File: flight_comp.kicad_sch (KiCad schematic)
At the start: 1 part, among them U1 STM32F405RGTx

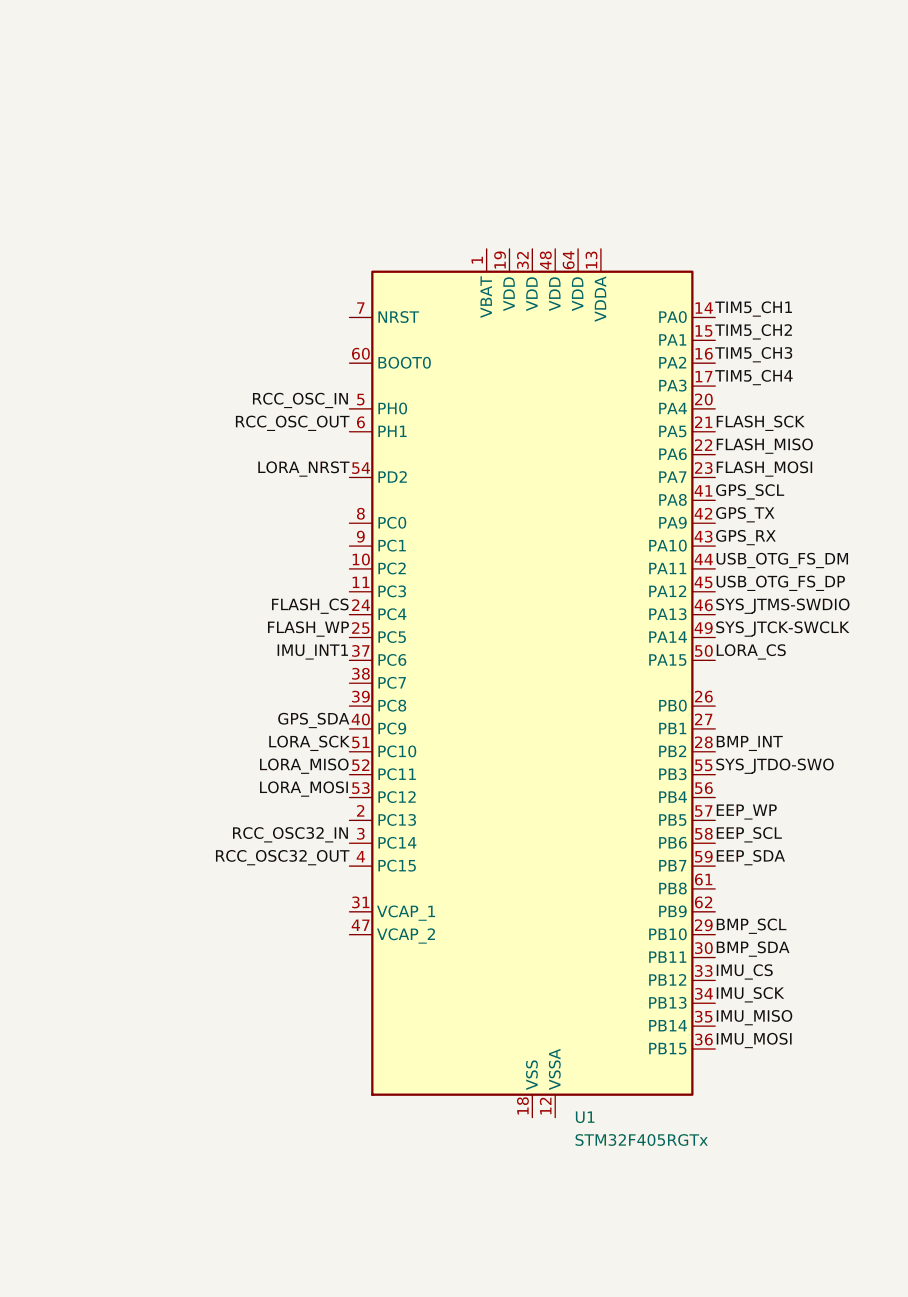
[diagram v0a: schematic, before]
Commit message: Sensors added
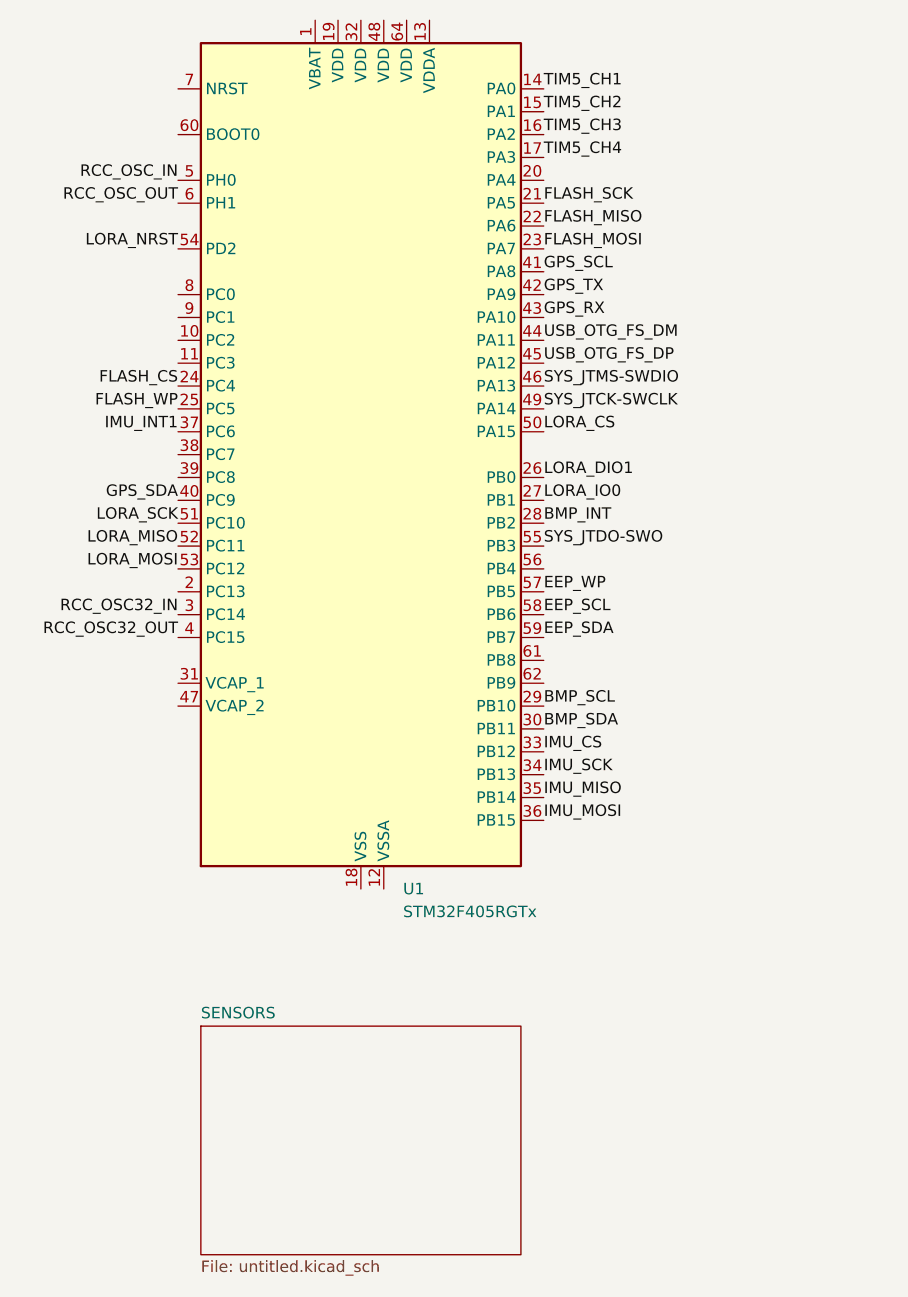
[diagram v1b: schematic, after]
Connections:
- net LORA_DIO1: now reaches U1.26 (PB0)
- net LORA_IO0: now reaches U1.27 (PB1)
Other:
- added sheet SENSORS (untitled.kicad_sch)
- moved on the sheet: U1
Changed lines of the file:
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@@
 	(paper "A4")
 	(label "TIM5_CH1"
-		(at 163.83 62.23 0)
+		(at 144.78 36.83 0)
+		(effects
+			(font
+				(size 1.27 1.27)
+			)
+			(justify left bottom)
+		)
+	)
+	(label "LORA_DIO1"
+		(at 144.78 80.01 0)
 		(effects
 			(font
@@
 	)
 	(label "EEP_SCL"
-		(at 163.83 120.65 0)
+		(at 144.78 95.25 0)
 		(effects
 			(font
@@
 	)
 	(label "TIM5_CH2"
-		(at 163.83 64.77 0)
+		(at 144.78 39.37 0)
 		(effects
 			(font
@@
 	)
 	(label "IMU_SCK"
-		(at 163.83 138.43 0)
+		(at 144.78 113.03 0)
 		(effects
 			(font
@@
 	)
 	(label "LORA_NRST"
-		(at 123.19 80.01 180)
+		(at 104.14 54.61 180)
 		(effects
 			(font
@@
 	)
 	(label "GPS_SDA"
-		(at 123.19 107.95 180)
+		(at 104.14 82.55 180)
 		(effects
 			(font
@@
 	)
 	(label "LORA_MOSI"
-		(at 123.19 115.57 180)
+		(at 104.14 90.17 180)
 		(effects
 			(font
@@
 	)
 	(label "USB_OTG_FS_DM"
-		(at 163.83 90.17 0)
+		(at 144.78 64.77 0)
 		(effects
 			(font
@@
 	)
 	(label "BMP_SDA"
-		(at 163.83 133.35 0)
+		(at 144.78 107.95 0)
 		(effects
 			(font
@@
 	)
 	(label "EEP_WP"
-		(at 163.83 118.11 0)
+		(at 144.78 92.71 0)
 		(effects
 			(font
@@
 	)
 	(label "GPS_TX"
-		(at 163.83 85.09 0)
+		(at 144.78 59.69 0)
 		(effects
 			(font
@@
 	)
 	(label "RCC_OSC_OUT"
-		(at 123.19 74.93 180)
+		(at 104.14 49.53 180)
 		(effects
 			(font
@@
 	)
 	(label "IMU_MOSI"
-		(at 163.83 143.51 0)
+		(at 144.78 118.11 0)
 		(effects
 			(font
@@
 	)
 	(label "IMU_CS"
-		(at 163.83 135.89 0)
+		(at 144.78 110.49 0)
 		(effects
 			(font
@@
 	)
 	(label "SYS_JTDO-SWO"
-		(at 163.83 113.03 0)
+		(at 144.78 87.63 0)
 		(effects
 			(font
@@
 	)
 	(label "TIM5_CH3"
-		(at 163.83 67.31 0)
+		(at 144.78 41.91 0)
 		(effects
 			(font
@@
 	)
 	(label "EEP_SDA"
-		(at 163.83 123.19 0)
+		(at 144.78 97.79 0)
 		(effects
 			(font
@@
 	)
 	(label "FLASH_CS"
-		(at 123.19 95.25 180)
+		(at 104.14 69.85 180)
 		(effects
 			(font
@@
 	)
 	(label "LORA_CS"
-		(at 163.83 100.33 0)
+		(at 144.78 74.93 0)
 		(effects
 			(font
@@
 	)
 	(label "GPS_SCL"
-		(at 163.83 82.55 0)
+		(at 144.78 57.15 0)
 		(effects
 			(font
@@
 	)
 	(label "RCC_OSC_IN"
-		(at 123.19 72.39 180)
+		(at 104.14 46.99 180)
 		(effects
 			(font
@@
 	)
 	(label "USB_OTG_FS_DP"
-		(at 163.83 92.71 0)
+		(at 144.78 67.31 0)
 		(effects
 			(font
@@
 	)
 	(label "FLASH_MOSI"
-		(at 163.83 80.01 0)
+		(at 144.78 54.61 0)
 		(effects
 			(font
@@
 	)
 	(label "SYS_JTCK-SWCLK"
-		(at 163.83 97.79 0)
+		(at 144.78 72.39 0)
 		(effects
 			(font
@@
 	)
 	(label "RCC_OSC32_OUT"
-		(at 123.19 123.19 180)
+		(at 104.14 97.79 180)
 		(effects
 			(font
@@
 	)
 	(label "FLASH_WP"
-		(at 123.19 97.79 180)
+		(at 104.14 72.39 180)
 		(effects
 			(font
@@
 	)
 	(label "SYS_JTMS-SWDIO"
-		(at 163.83 95.25 0)
+		(at 144.78 69.85 0)
 		(effects
 			(font
@@
 	)
 	(label "RCC_OSC32_IN"
-		(at 123.19 120.65 180)
+		(at 104.14 95.25 180)
 		(effects
 			(font
@@
 	)
 	(label "BMP_INT"
-		(at 163.83 110.49 0)
+		(at 144.78 85.09 0)
 		(effects
 			(font
@@
 	)
 	(label "GPS_RX"
-		(at 163.83 87.63 0)
+		(at 144.78 62.23 0)
 		(effects
 			(font
@@
 	)
 	(label "BMP_SCL"
-		(at 163.83 130.81 0)
+		(at 144.78 105.41 0)
 		(effects
 			(font
@@
 	)
 	(label "TIM5_CH4"
-		(at 163.83 69.85 0)
+		(at 144.78 44.45 0)
 		(effects
 			(font
@@
 	)
 	(label "IMU_MISO"
-		(at 163.83 140.97 0)
+		(at 144.78 115.57 0)
 		(effects
 			(font
@@
 	)
 	(label "FLASH_SCK"
-		(at 163.83 74.93 0)
+		(at 144.78 49.53 0)
+		(effects
+			(font
+				(size 1.27 1.27)
+			)
+			(justify left bottom)
+		)
+	)
+	(label "LORA_IO0"
+		(at 144.78 82.55 0)
 		(effects
 			(font
@@
 	)
 	(label "IMU_INT1"
-		(at 123.19 100.33 180)
+		(at 104.14 74.93 180)
 		(effects
 			(font
@@
 	)
 	(label "LORA_MISO"
-		(at 123.19 113.03 180)
+		(at 104.14 87.63 180)
 		(effects
 			(font
@@
 	)
 	(label "FLASH_MISO"
-		(at 163.83 77.47 0)
+		(at 144.78 52.07 0)
 		(effects
 			(font
@@
 	)
 	(label "LORA_SCK"
-		(at 123.19 110.49 180)
+		(at 104.14 85.09 180)
 		(effects
 			(font
@@
 	(symbol
 		(lib_id "MCU_ST_STM32F4:STM32F405RGTx")
-		(at 143.51 102.87 0)
+		(at 124.46 77.47 0)
 		(unit 1)
 		(exclude_from_sim no)
@@
 		(fields_autoplaced yes)
 		(property "Reference" "U1"
-			(at 148.1933 151.13 0)
+			(at 129.1433 125.73 0)
 			(effects
 				(font
@@
 		)
 		(property "Value" "STM32F405RGTx"
-			(at 148.1933 153.67 0)
+			(at 129.1433 128.27 0)
 			(effects
 				(font
@@
 		)
 		(property "Footprint" "Package_QFP:LQFP-64_10x10mm_P0.5mm"
-			(at 125.73 148.59 0)
+			(at 106.68 123.19 0)
 			(effects
 				(font
@@
 		)
 		(property "Datasheet" "https://www.st.com/resource/en/datasheet/stm32f405rg.pdf"
-			(at 143.51 102.87 0)
+			(at 124.46 77.47 0)
 			(effects
 				(font
@@
 		)
 		(property "Description" "STMicroelectronics Arm Cortex-M4 MCU, 1024KB flash, 192KB RAM, 168 MHz, 1.8-3.6V, 51 GPIO, LQFP64"
-			(at 143.51 102.87 0)
+			(at 124.46 77.47 0)
 			(effects
 				(font
@@
 				)
 			)
+		)
+	)
+	(sheet
+		(at 106.68 140.97)
+		(size 35.56 25.4)
+		(exclude_from_sim no)
+		(in_bom yes)
+		(on_board yes)
+		(dnp no)
+		(fields_autoplaced yes)
+		(stroke
+			(width 0.1524)
+			(type solid)
+		)
+		(fill
+			(color 0 0 0 0.0000)
+		)
+		(property "Sheetname" "SENSORS"
+			(at 106.68 140.2584 0)
+			(effects
+				(font
+					(size 1.27 1.27)
+				)
+				(justify left bottom)
+			)
+		)
+		(property "Sheetfile" "untitled.kicad_sch"
+			(at 106.68 166.9546 0)
+			(effects
+				(font
+					(size 1.27 1.27)
+				)
+				(justify left top)
+			)
+		)
+		(instances
+			(project "flight_comp"
+				(path "/99100214-bcab-4638-96e7-2342f837a8e5"
+					(page "2")
+				)
+			)
